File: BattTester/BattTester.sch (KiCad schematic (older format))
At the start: 28 parts, among them J1 Battery, J2 SD_Card, J3 PWR, J4 UPDI, Q1 IRLZ44N, Q2 IRF4905, U1 LTC1286CN8, U2 ATtiny1624-SS, U3 LD1086DT33, U4 LM358AN

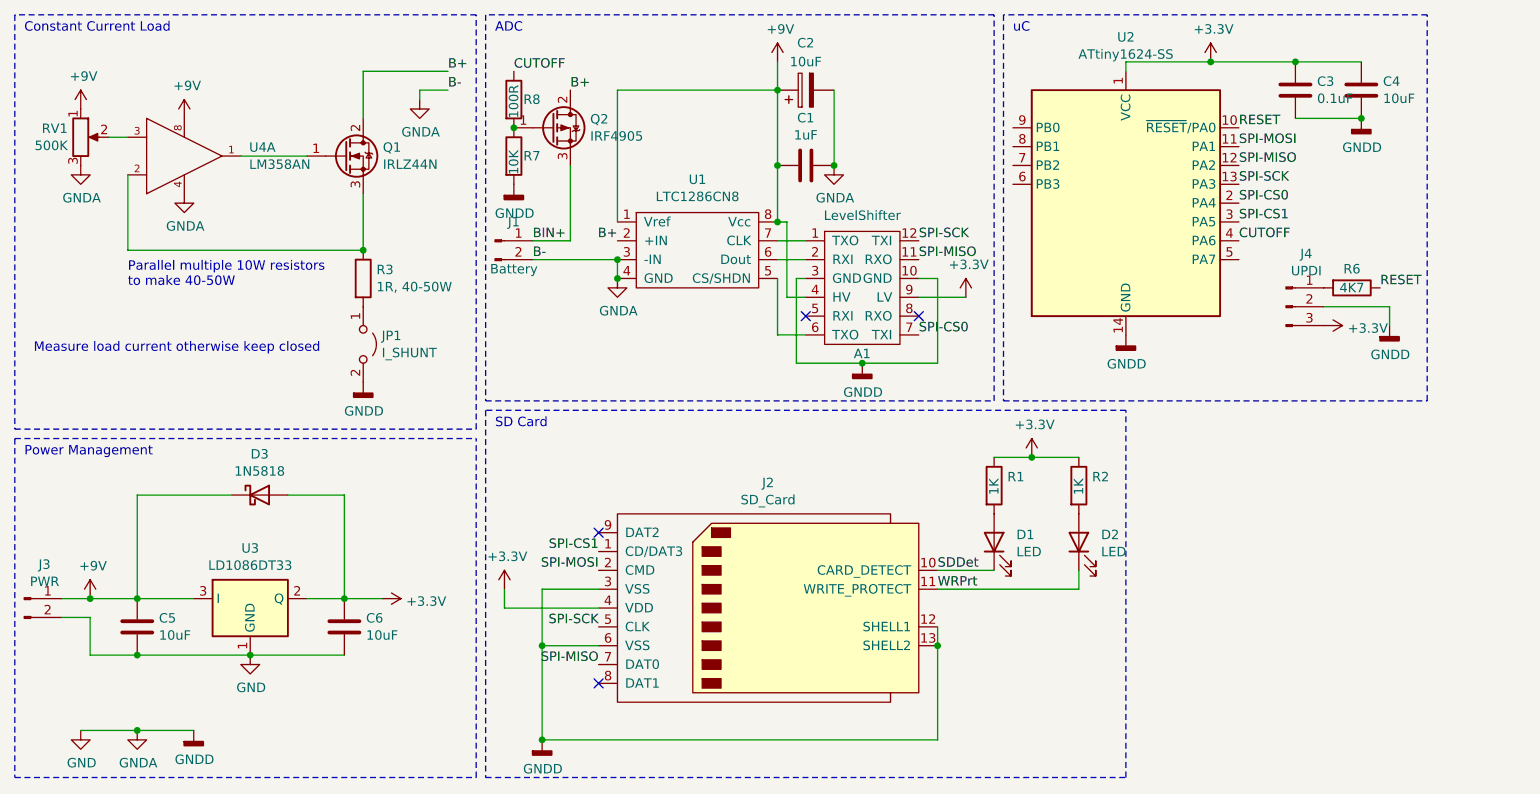
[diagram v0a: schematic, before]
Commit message: Fix #1
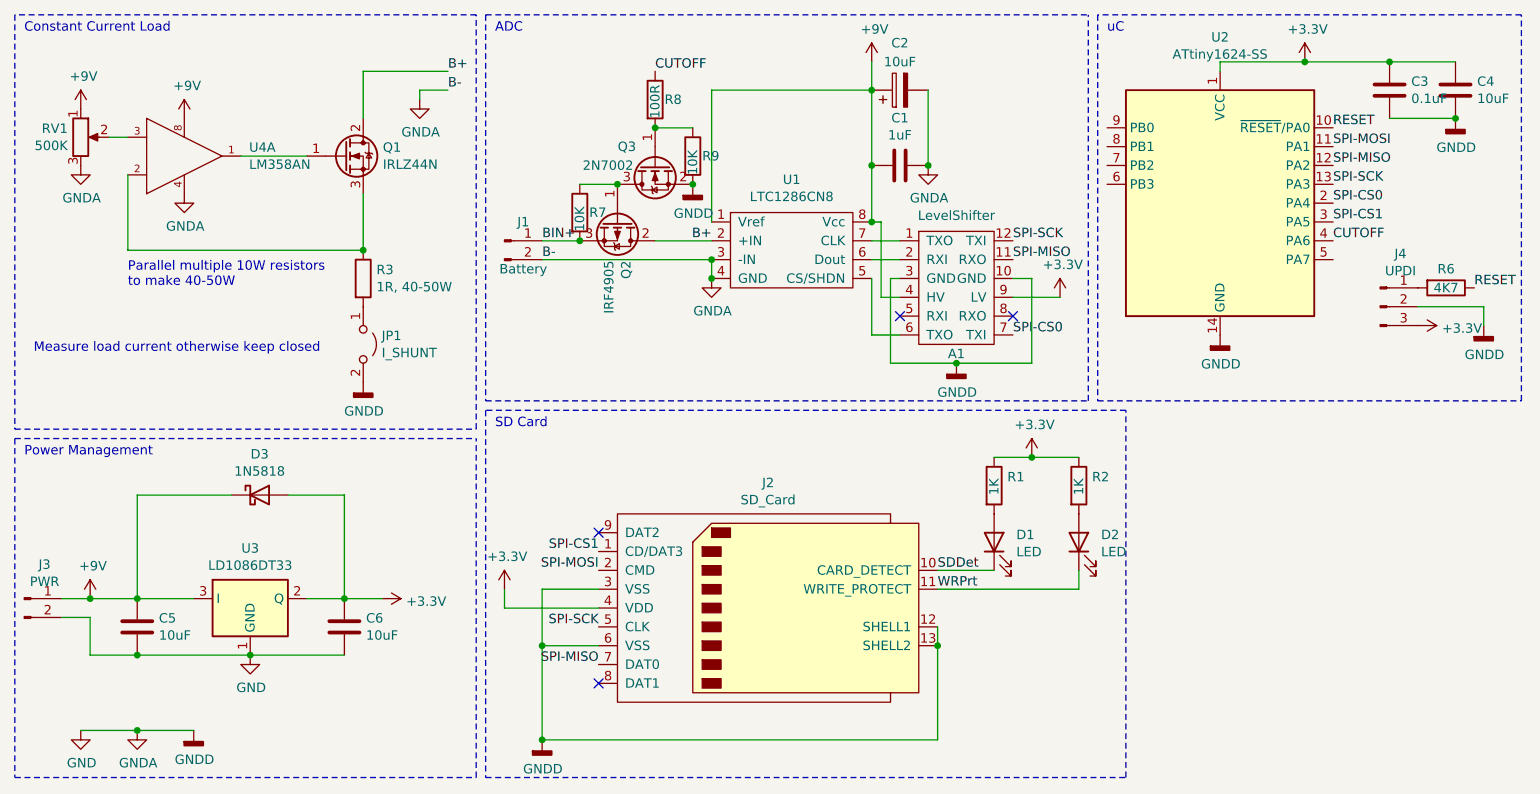
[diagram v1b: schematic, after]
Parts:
- added Q3: 2N7002, Package_TO_SOT_SMD:SOT-23, symbol Transistor_FET:2N7002
- added R9: 10K, Resistor_SMD:R_1206_3216Metric_Pad1.30x1.75mm_HandSolder, symbol Device:R
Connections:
- net BIN+: now also R7.2
- net GND: now also Q3.2 (S), R9.2; no longer R7.2
- net at Q2.1 (G), R7.1: now also Q3.3 (D); no longer R8.2
- new net: Q3.1 (G), R8.2, R9.1
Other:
- moved on the sheet: A1, C1, C2, C3, C4, J1, J4, Q2, R6, R7, R8, U1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
